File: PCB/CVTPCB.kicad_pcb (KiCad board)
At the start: 2 copper layers, 61 x 83.5 mm, 24 parts, among them J1 Infared, J2 TMP36, J3 Infared, J4 2x1, J5 TMP36, J7 SystemInput

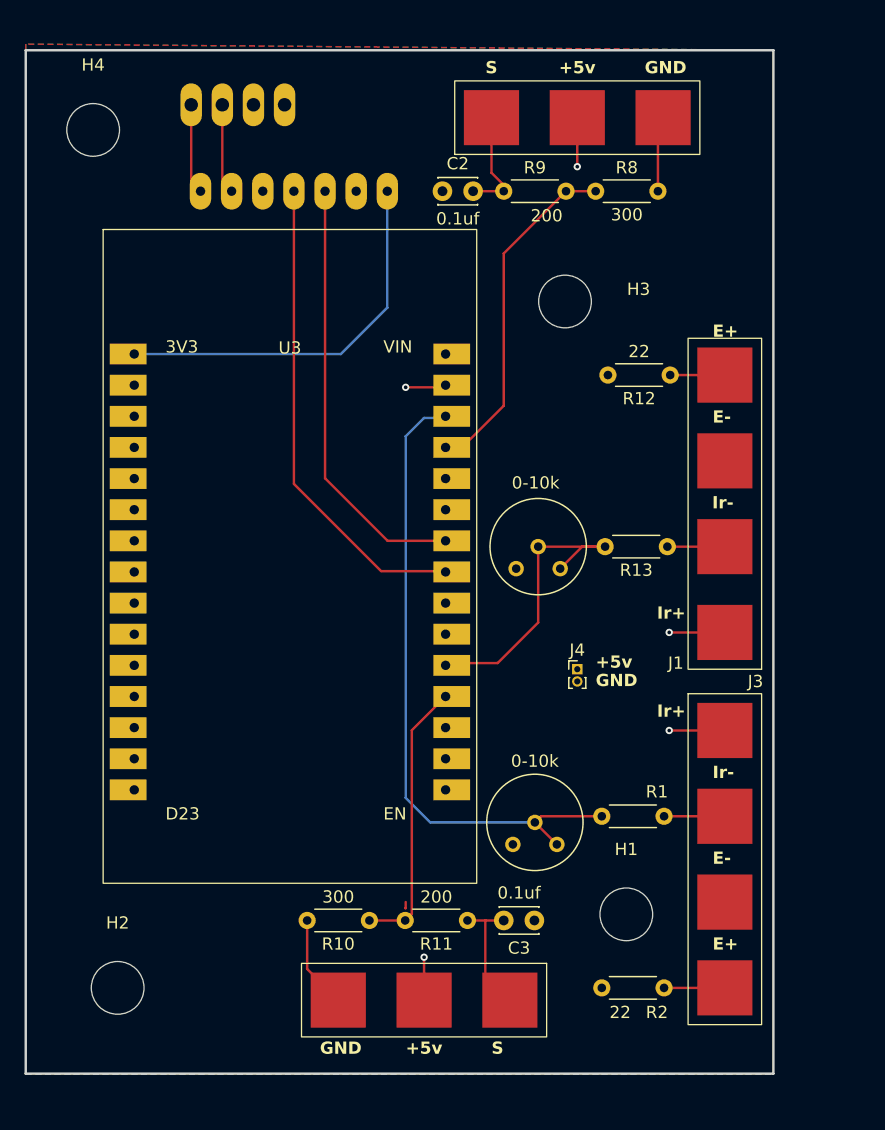
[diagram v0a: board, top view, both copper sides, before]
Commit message: Add files via upload
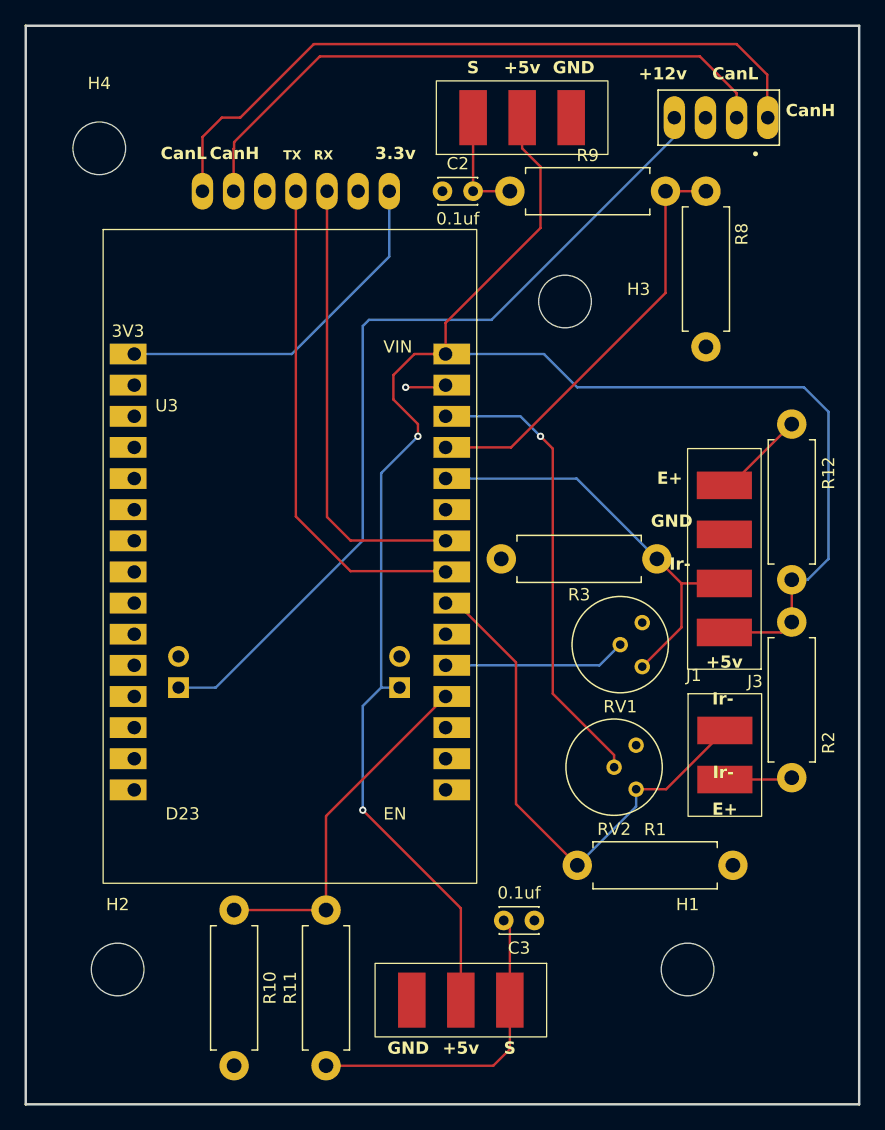
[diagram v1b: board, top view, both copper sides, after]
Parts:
- removed R13: R, Resistor_THT:R_Axial_DIN0204_L3.6mm_D1.6mm_P5.08mm_Horizontal
- added R3: R, Resistor_THT:R_Axial_DIN0411_L9.9mm_D3.6mm_P12.70mm_Horizontal, F.Cu at (151.5, 96.0)
- J4: value 2x1 -> Conn_01x04_Pin; footprint Connector_PinHeader_1.00mm:PinHeader_1x02_P1.00mm_Vertical -> CVT:PowerBoard; moved to B.Cu
- J7: moved to F.Cu
- R1, R10, R11, R12, R2, R8, R9: footprint Resistor_THT:R_Axial_DIN0204_L3.6mm_D1.6mm_P5.08mm_Horizontal -> Resistor_THT:R_Axial_DIN0411_L9.9mm_D3.6mm_P12.70mm_Horizontal
- moved J7 39.1 mm to (156.5, 60.0), turned to 0 degrees
- moved R2 20.1 mm to (162.5, 113.8), turned to 90 degrees
- moved R11 16.5 mm to (124.5, 137.3), turned to 90 degrees
- moved R10 11.1 mm to (117.0, 124.7), turned to -90 degrees
- moved R12 10.7 mm to (162.5, 85.0), turned to -90 degrees
- moved RV2 10.4 mm to (149.8, 111.2), turned to 180 degrees
- moved J4 9.54 mm to (135.5, 105.2), turned to 90 degrees
- moved R8 9.00 mm to (155.5, 66.0), turned to -90 degrees
- moved R1 8.13 mm to (145.0, 121.0), turned to 0 degrees
- moved RV1 8.01 mm to (150.3, 101.2), turned to 180 degrees
- moved H1 6.73 mm to (154.0, 129.5)
- moved H4 1.58 mm to (106.0, 62.5)
- moved H2 1.50 mm to (107.5, 129.5)
- moved J2 1.50 mm to (130.5, 60.0)
- moved R9 0.50 mm to (139.5, 66.0)
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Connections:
- J1 pad 2: Net-(J1-IR-) -> /IrOut1
- J3 pad 2: Net-(J3-IR-) -> /IrOut2
- J7 pad 4: +12V -> /+12v
- R1 pad 1: Net-(J1-IR-) -> /IrOut1
- R1 pad 2: /Ir2 -> GND
- RV1 pad 1: /Ir1 -> GND
- RV1 pad 3: GND -> /IrOut2
- RV2 pad 1: /Ir2 -> GND
- RV2 pad 3: GND -> /IrOut1
- U3 pad 22: unconnected-(U3-D33-Pad22) -> /IrOut1
- U3 pad 26: unconnected-(U3-D14-Pad26) -> /IrOut2
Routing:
- net +5V: track 16.6 -> 144.8 mm, vias 4 -> 2
- net /+12v: track 0.00 -> 70.9 mm
- net /CanL: track 7.36 -> 58.2 mm
- net /IrOut1: track 0.00 -> 43.8 mm
- net /CanH: track 7.36 -> 51.2 mm
- net /IrOut2: track 0.00 -> 34.4 mm
- net Net-(J5-s): track 10.3 -> 26.3 mm
- net /Ir2: track 53.0 -> 37.9 mm, vias 0 -> 1
- net GND: track 17.1 -> 3.33 mm
- net /Ir1: track 25.1 -> 14.9 mm
- net /TMP36_2: track 28.2 -> 34.8 mm
- net /TMP36_1: track 22.6 -> 29.0 mm
- net Net-(J1-IR-): track 4.96 -> 0.00 mm
- net Net-(J3-IR-): track 4.69 -> 0.00 mm
- net Net-(J3-E+): track 4.46 -> 7.57 mm
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- removed copper zone on B.Cu, net +5V
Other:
- board size 61 x 83.5 mm -> 68 x 88 mm
- board text added: "12+"
- board text added: "CanH"
- board text added: "CanL"
- board text added: "RX"
- board text added: "TX"
- board text removed: "E-"
- board text removed: "Ir+"
